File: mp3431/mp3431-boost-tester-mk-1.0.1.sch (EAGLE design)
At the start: 34 parts, among them J1 AVR_SPI_PRG_6SMD-1.27MM, U1 MP3431, U2 INA190RSW, U3 TLV70028DCK, U4 ATTINY45TINY85-20-QFN

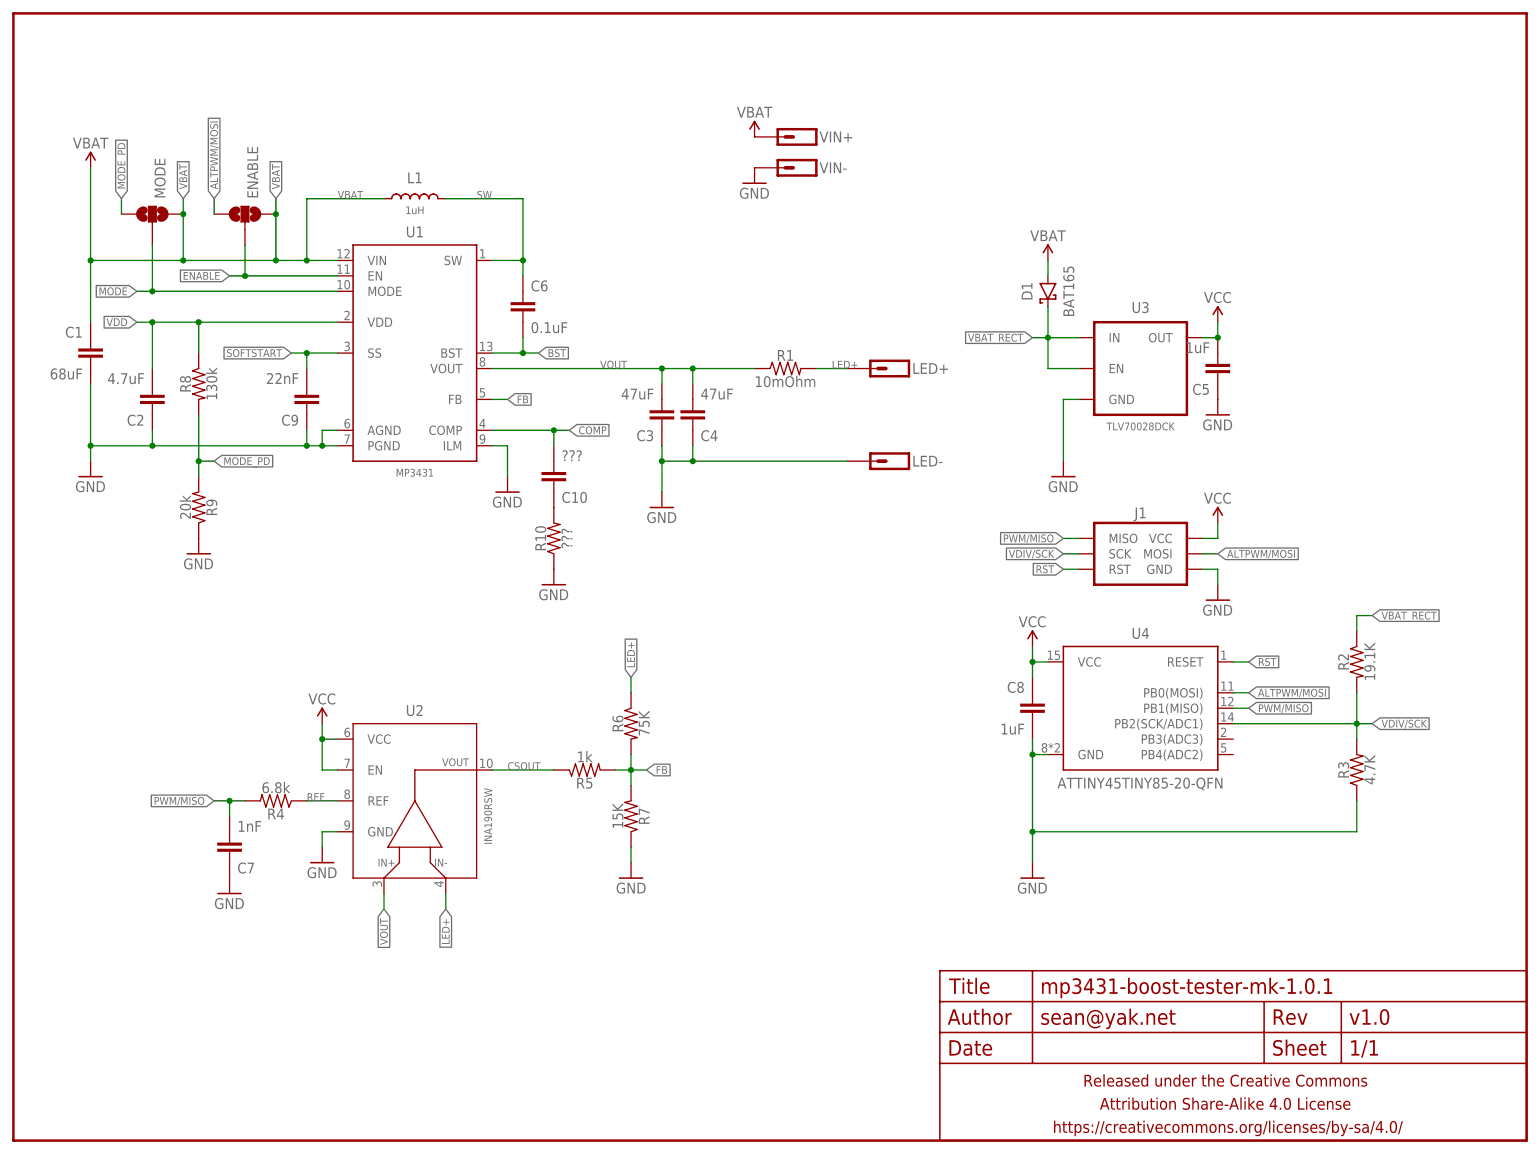
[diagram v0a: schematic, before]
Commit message: more wip
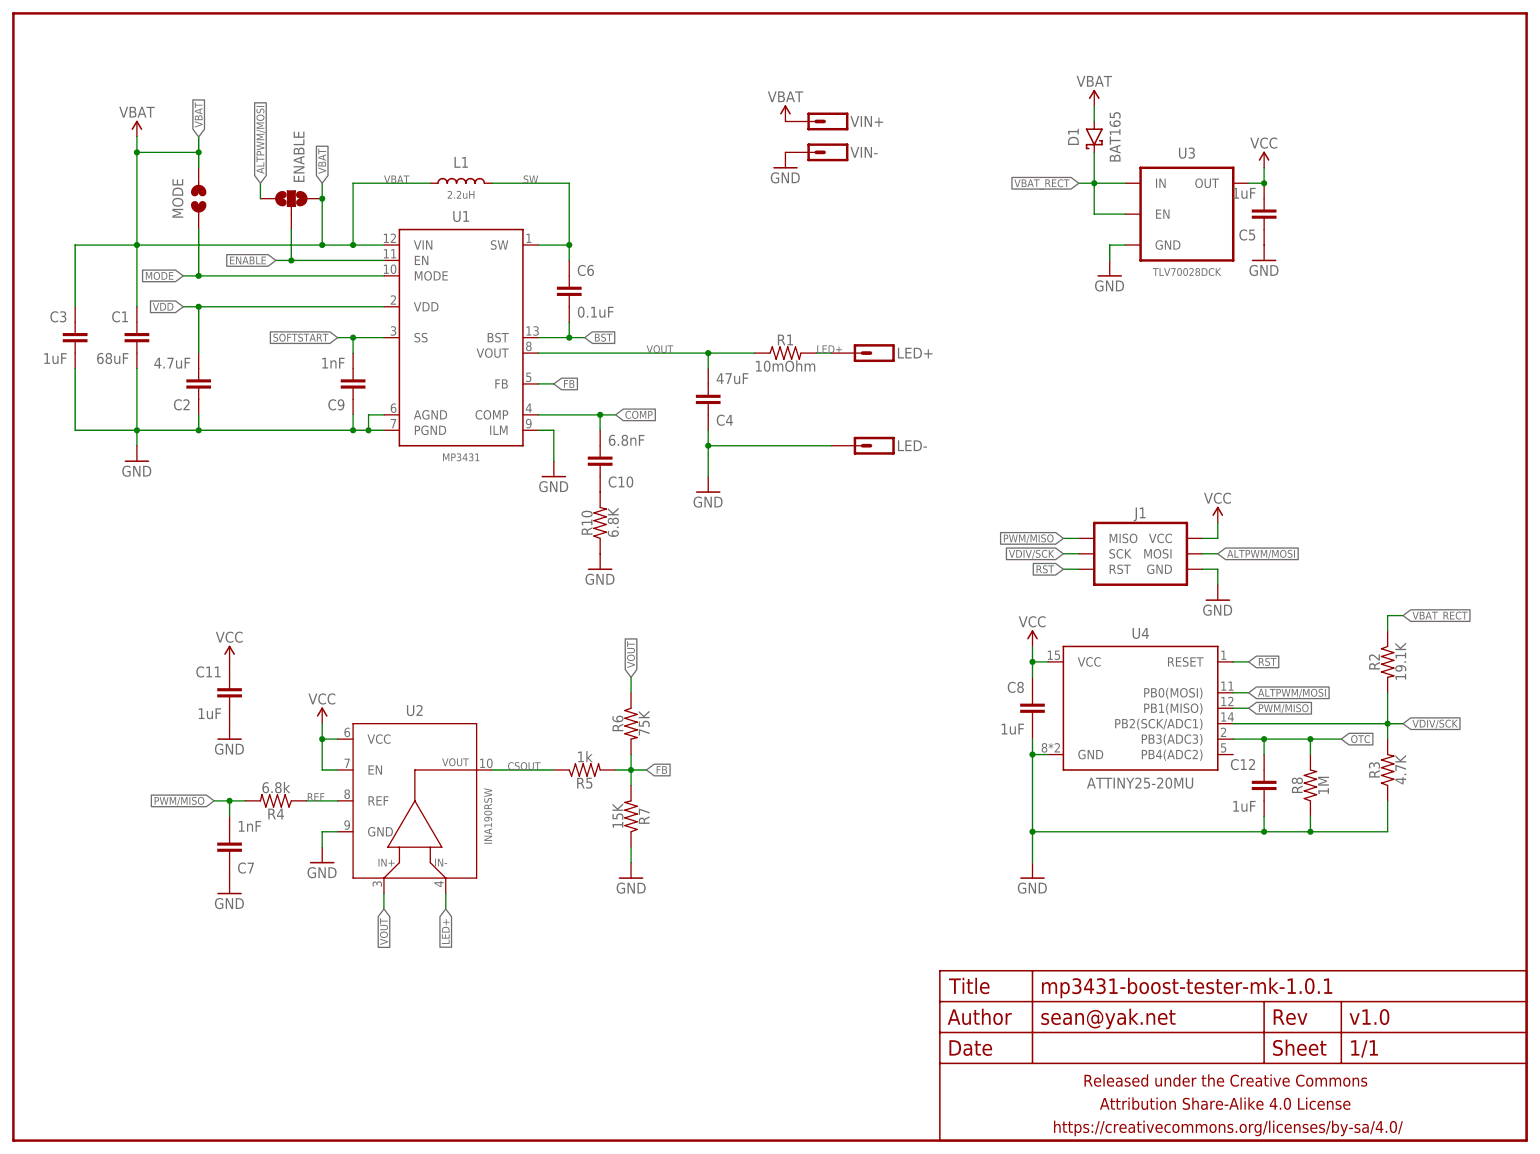
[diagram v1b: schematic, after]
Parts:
- removed R9: 20k, a_parts:RESISTORR0402
- added C11, C12: 1uF, a_parts:CAPACITOR-CERAMICC0402
- C1, C4: device a_parts:CAPACITOR-CERAMICC1206 -> a_parts:CAPACITOR-CERAMICC1210
- C10: value ??? -> 6.8nF
- C3: value 47uF -> 1uF; device a_parts:CAPACITOR-CERAMICC1206 -> a_parts:CAPACITOR-CERAMICC0402
- C9: value 22nF -> 1nF
- J1: value AVR_SPI_PRG_6SMD-1.27MM -> AVR_SPI_PRG_6PTH; device a_parts:AVR_SPI_PRG_6SMD-1.27MM -> a_parts:AVR_SPI_PRG_6PTH
- L1: value 1uH -> 2.2uH
- MODE: value JUMPER-PAD-3-NOSMALL_BOX_SILK -> JUMPER-PAD-2-NOYES_SILK; device a_parts:JUMPER-PAD-3-NOSMALL_BOX_SILK -> a_parts:JUMPER-PAD-2-NOYES_SILK
- R10: value ??? -> 6.8K
- R8: value 130k -> 1M
- U4: value ATTINY45TINY85-20-QFN -> ATTINY25-20MU
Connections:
- removed net MODE_PD: MODE.3, R8.2, R9.2
- new net OTC: C12.1, R8.2, U4.PB3(ADC3)
- net GND: now also C11.2, C12.2, C3.2, R8.1; no longer C3.1, R9.1
- net LED+: no longer R6.1
- net MODE: now also MODE.1; no longer MODE.2
- net VBAT: now also C3.1, MODE.2; no longer MODE.1
- net VCC: now also C11.1
- net VDD: no longer R8.1
- net VOUT: now also R6.1; no longer C3.2
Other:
- moved on the sheet: C1, C10, C2, C3, C4, C5, C6, C9, D1, ENABLE, L1, LED+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
